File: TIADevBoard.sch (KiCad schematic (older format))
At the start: 23 parts, among them J1 Screw_Terminal_01x02, J2 Conn_Coaxial, J3 Conn_Coaxial, J4 Conn_02x03_Counter_Clockwise, J5 Conn_Coaxial, U2 OPA2387, U3 ADP3330-3.3

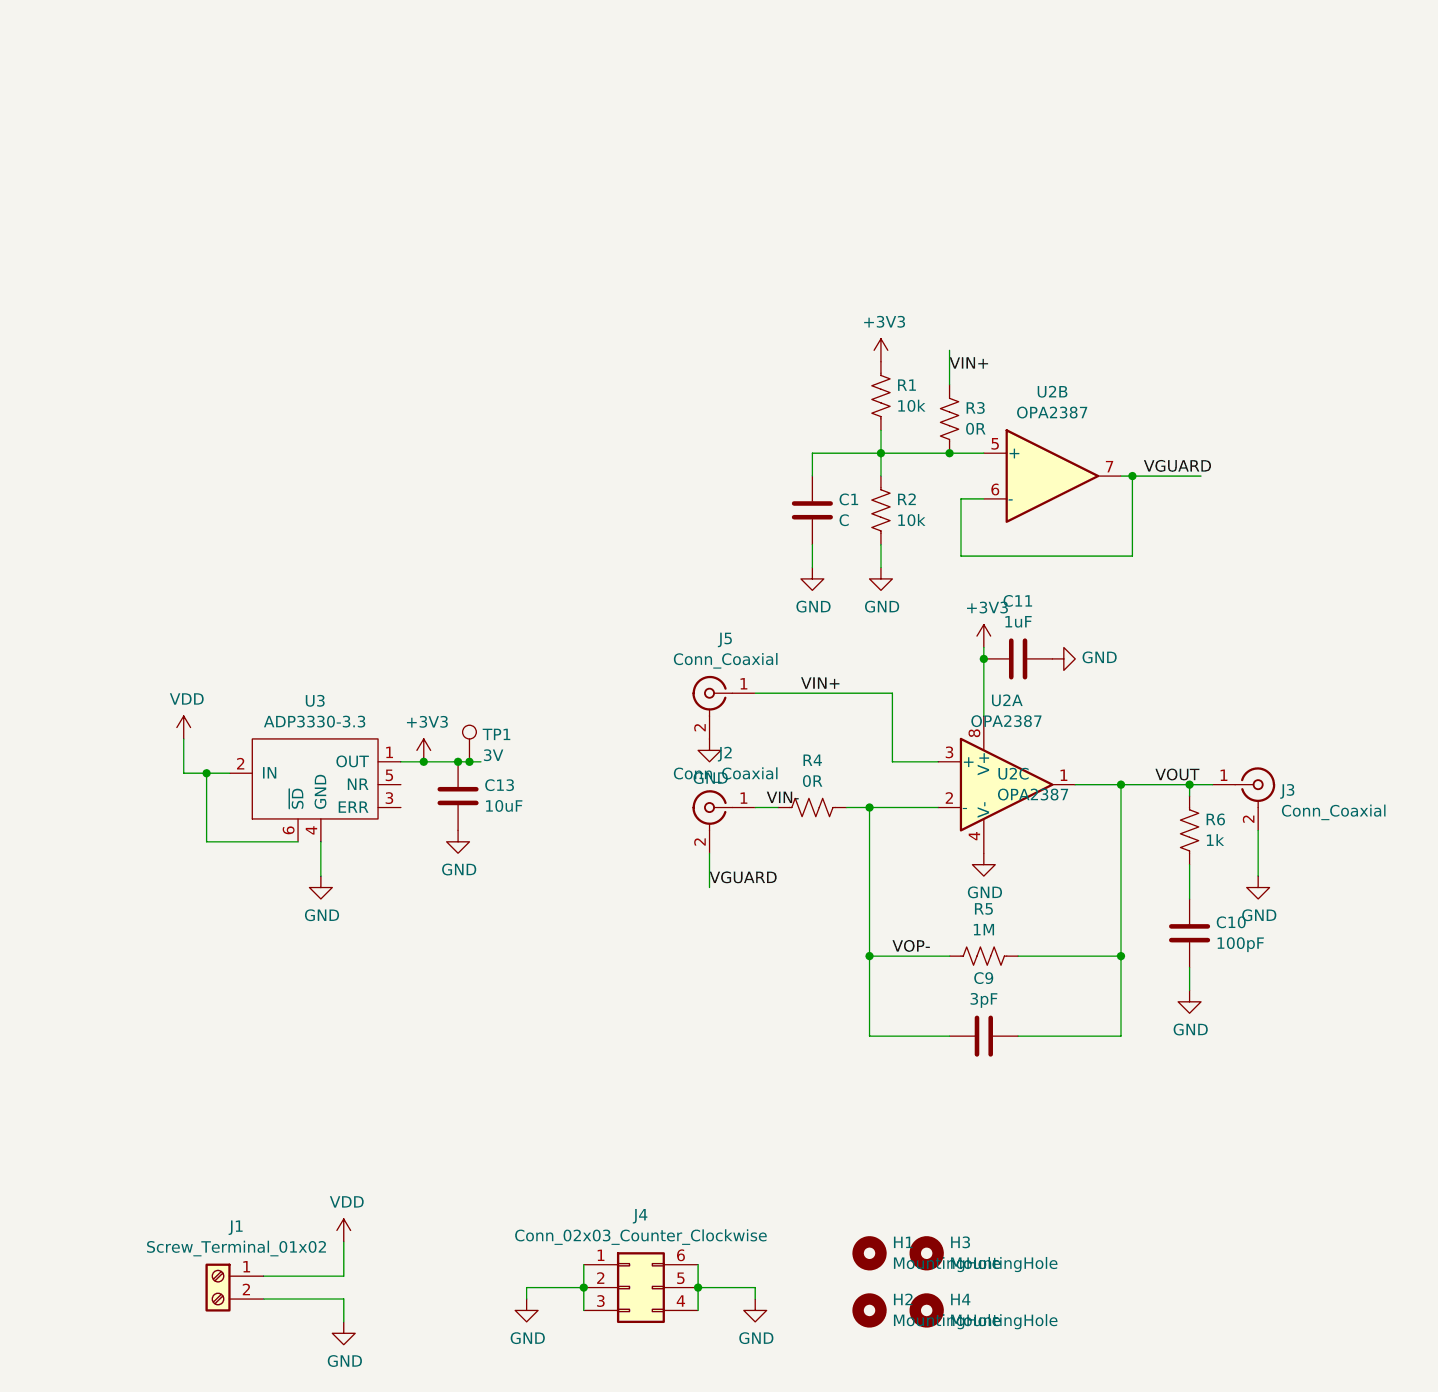
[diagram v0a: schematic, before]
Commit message: added gerbers for version 5
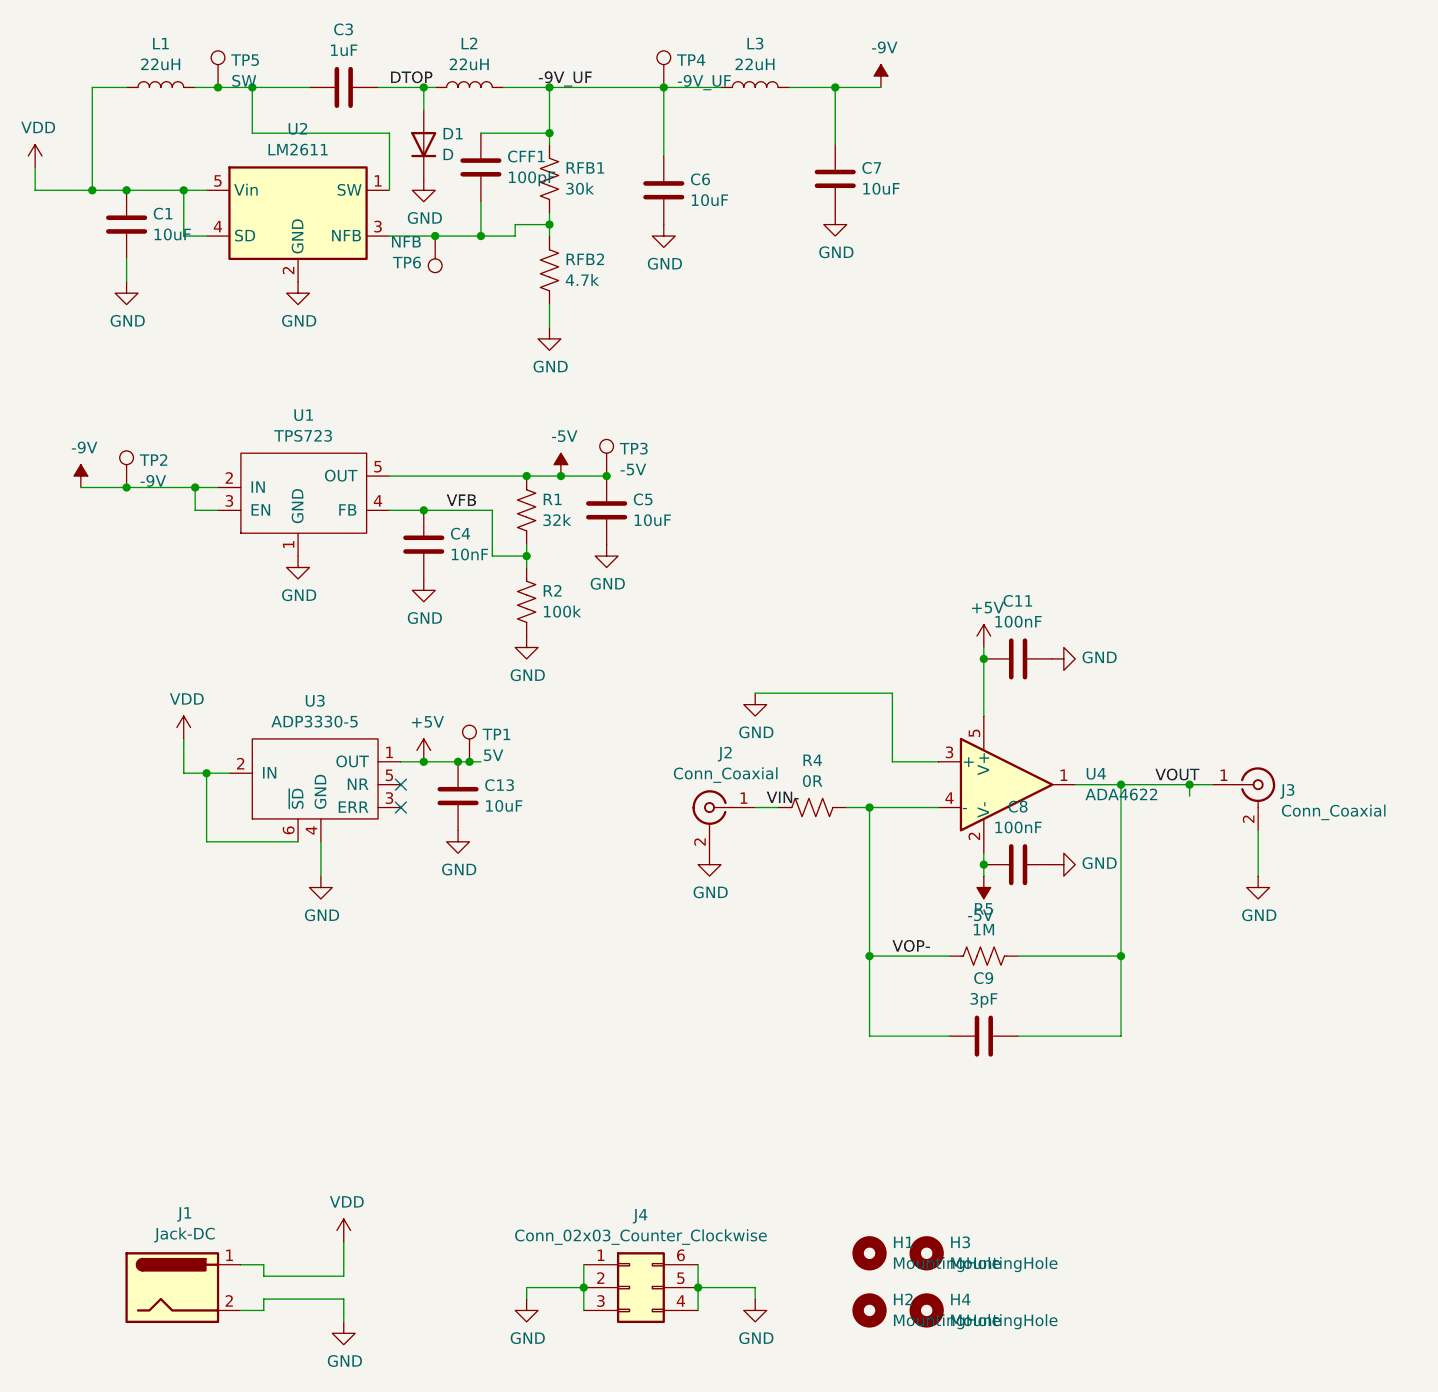
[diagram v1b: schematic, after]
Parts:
- removed C10: 100pF, Capacitor_SMD:C_0805_2012Metric_Pad1.15x1.40mm_HandSolder, symbol Device:C
- removed J1: Screw_Terminal_01x02, TerminalBlock:TerminalBlock_Altech_AK300-2_P5.00mm, symbol Connector:Screw_Terminal_01x02
- removed J5: Conn_Coaxial, my_library_foot:CON-SMA-EDGE-S, symbol Connector:Conn_Coaxial
- removed R3: 0R, Resistor_SMD:R_0805_2012Metric_Pad1.15x1.40mm_HandSolder, symbol Device:R_US
- removed R6: 1k, Resistor_SMD:R_0805_2012Metric_Pad1.15x1.40mm_HandSolder, symbol Device:R_US
- removed U2: OPA2387, Package_SO:VSSOP-8_3.0x3.0mm_P0.65mm, symbol my_library:OPA2387
- added C3: 1uF, Capacitor_SMD:C_0805_2012Metric_Pad1.15x1.40mm_HandSolder, symbol Device:C
- added C4: 10nF, Capacitor_SMD:C_0805_2012Metric_Pad1.15x1.40mm_HandSolder, symbol Device:C
- added C5, C6, C7: 10uF, Capacitor_SMD:C_0805_2012Metric_Pad1.15x1.40mm_HandSolder, symbol Device:C
- added C8: 100nF, Capacitor_SMD:C_0805_2012Metric_Pad1.15x1.40mm_HandSolder, symbol Device:C
- added CFF1: 100pF, Capacitor_SMD:C_0805_2012Metric_Pad1.15x1.40mm_HandSolder, symbol Device:C
- added D1: D, Diode_SMD:D_SOD-323_HandSoldering, symbol Device:D
- added J1: Jack-DC, Connector_BarrelJack:BarrelJack_Horizontal, symbol Connector:Jack-DC
- added L1, L2, L3: 22uH, Inductor_SMD:L_0805_2012Metric_Pad1.15x1.40mm_HandSolder, symbol Device:L
- added RFB1: 30k, Resistor_SMD:R_0805_2012Metric_Pad1.15x1.40mm_HandSolder, symbol Device:R_US
- added RFB2: 4.7k, Resistor_SMD:R_0805_2012Metric_Pad1.15x1.40mm_HandSolder, symbol Device:R_US
- added TP2: -9V, my_library_foot:TestPoint_Keystone_5000-5004_Miniature, symbol Connector:TestPoint
- added TP3: -5V, my_library_foot:TestPoint_Keystone_5000-5004_Miniature, symbol Connector:TestPoint
- added TP4: -9V_UF, my_library_foot:TestPoint_Keystone_5000-5004_Miniature, symbol Connector:TestPoint
- added TP5: SW, my_library_foot:TestPoint_Keystone_5000-5004_Miniature, symbol Connector:TestPoint
- added TP6: NFB, my_library_foot:TestPoint_Keystone_5000-5004_Miniature, symbol Connector:TestPoint
- added U1: TPS723, Package_TO_SOT_SMD:SOT-23-5_HandSoldering, symbol my_library:TPS723
- added U2: LM2611, Package_TO_SOT_SMD:SOT-23-5_HandSoldering, symbol my_library:LM2611
- added U4: ADA4622, Package_TO_SOT_SMD:SOT-23-5_HandSoldering, symbol my_library:ADA4622
- C1: value C -> 10uF
- C11: value 1uF -> 100nF
- R1: value 10k -> 32k
- R2: value 10k -> 100k
- TP1: value 3V -> 5V
- U3: value ADP3330-3.3 -> ADP3330-5
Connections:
- net labels added: +5V, -5V, -9V, -9V_UF, DTOP, VFB
- net labels removed: +3V3, VGUARD, VIN+
- wire segments 61 -> 101
- no-connect marks 0 -> 2
